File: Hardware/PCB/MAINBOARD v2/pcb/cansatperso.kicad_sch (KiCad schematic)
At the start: 40 parts, among them IC1 2536030320001, J2 47309-2651, SW1 RSTBTN, U1 STM32G431CBUx, U3 BMP581, Y1 Crystal_GND24_Small

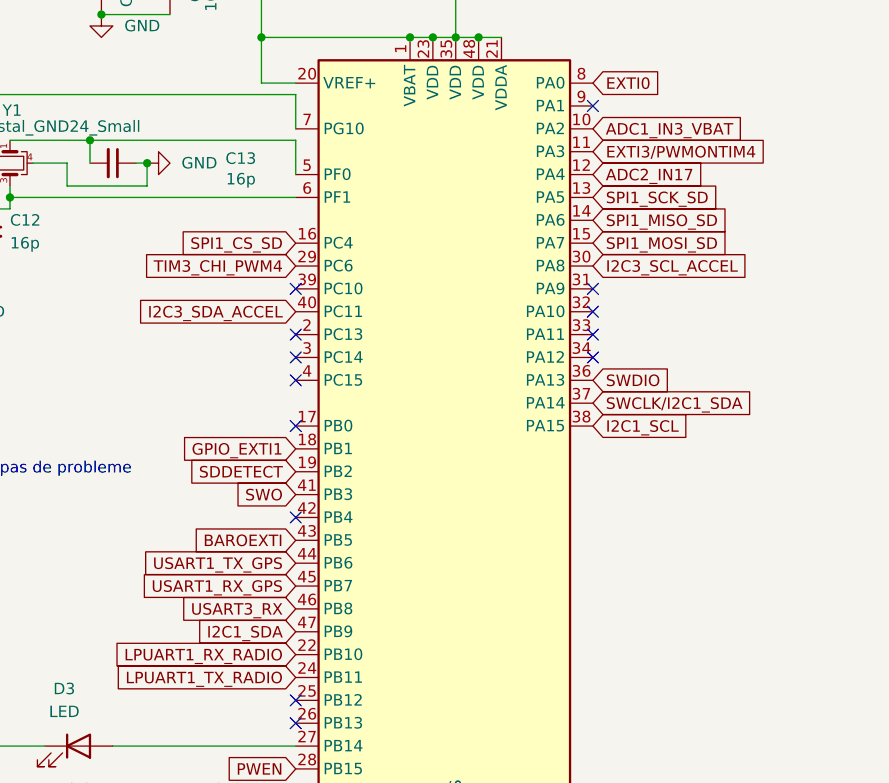
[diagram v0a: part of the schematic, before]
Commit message: pcb
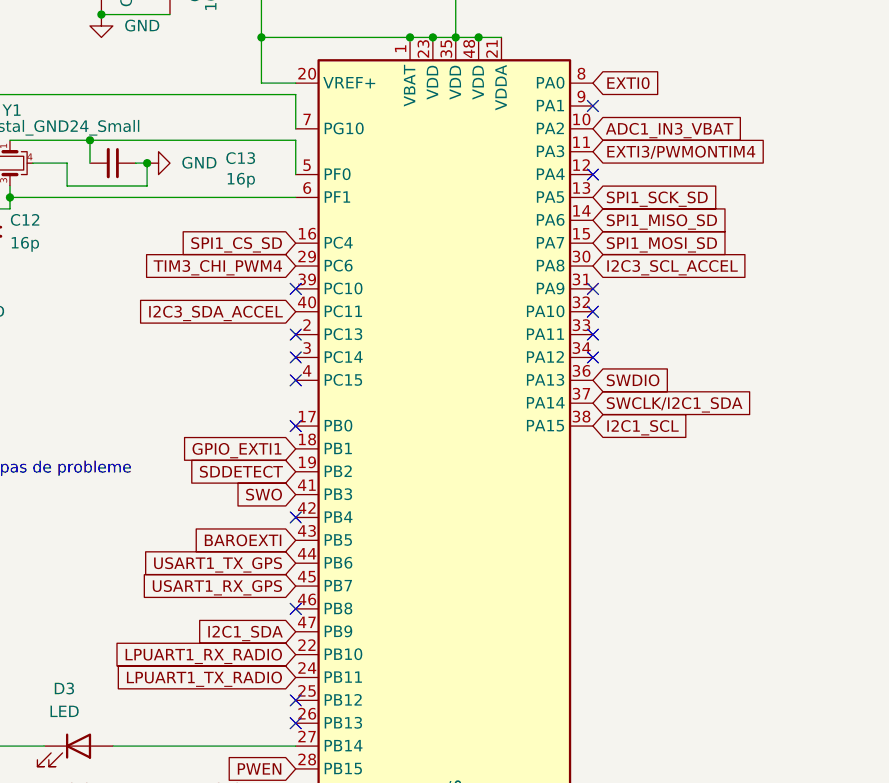
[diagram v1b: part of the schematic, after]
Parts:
- IC1: footprint WSEN-ISDS:2536030320001 -> WSEN ISDS:2536030320001
- J2: footprint molexmicrosd:47309-2651 -> micro sd:47309-2651
- U3: footprint bmp581:BMP581 -> BMP581:BMP581
- Y1: footprint crystalmulticomp:MCSJK7U1200101080B10 -> crystal:MCSJK7U1200101080B10
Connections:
- net ADC2_IN17: no longer names the net of U1.12 (PA4)
- net USART3_RX: no longer names the net of U1.46 (PB8)
- no-connect marks 18 -> 20
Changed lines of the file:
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@@
 	)
 	(no_connect
+		(at 119.38 88.9)
+	)
+	(no_connect
 		(at 86.36 127)
 	)
@@
 	)
 	(no_connect
+		(at 86.36 137.16)
+	)
+	(no_connect
 		(at 119.38 106.68)
 	)
@@
 		)
 	)
-	(global_label "ADC2_IN17"
-		(shape input)
-		(at 119.38 88.9 0)
-		(fields_autoplaced yes)
-		(effects
-			(font
-				(size 1.27 1.27)
-			)
-			(justify left)
-		)
-		(property "Intersheetrefs" "${INTERSHEET_REFS}"
-			(at 132.5252 88.9 0)
-			(effects
-				(font
-					(size 1.27 1.27)
-				)
-				(justify left)
-				(hide yes)
-			)
-		)
-	)
 	(global_label "EXTI0"
 		(shape input)
@@
 		)
 	)
-	(global_label "USART3_RX"
-		(shape input)
-		(at 86.36 137.16 180)
-		(fields_autoplaced yes)
-		(effects
-			(font
-				(size 1.27 1.27)
-			)
-			(justify right)
-		)
-		(property "Intersheetrefs" "${INTERSHEET_REFS}"
-			(at 72.852 137.16 0)
-			(effects
-				(font
-					(size 1.27 1.27)
-				)
-				(justify right)
-				(hide yes)
-			)
-		)
-	)
 	(global_label "PWEN"
 		(shape input)
@@
 			)
 		)
-		(property "Footprint" "bmp581:BMP581"
+		(property "Footprint" "BMP581:BMP581"
 			(at 135.89 319.71 0)
 			(effects
@@
 			)
 		)
-		(property "Footprint" "molexmicrosd:47309-2651"
+		(property "Footprint" "micro sd:47309-2651"
 			(at 308.61 146.99 0)
 			(effects
@@
 			)
 		)
-		(property "Footprint" "WSEN-ISDS:2536030320001"
+		(property "Footprint" "WSEN ISDS:2536030320001"
 			(at 321.31 261.29 0)
 			(effects
@@
 			)
 		)
-		(property "Footprint" "crystalmulticomp:MCSJK7U1200101080B10"
+		(property "Footprint" "crystal:MCSJK7U1200101080B10"
 			(at 54.61 87.63 0)
 			(effects
